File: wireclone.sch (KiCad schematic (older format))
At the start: 2 parts, among them P2 CONN_01X03, P3 CONN_01X03

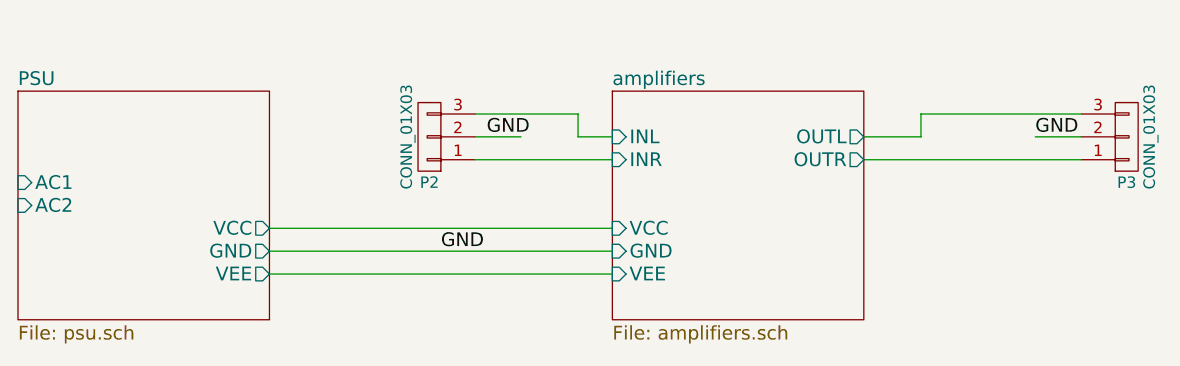
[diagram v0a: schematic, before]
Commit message: complete layout drafted
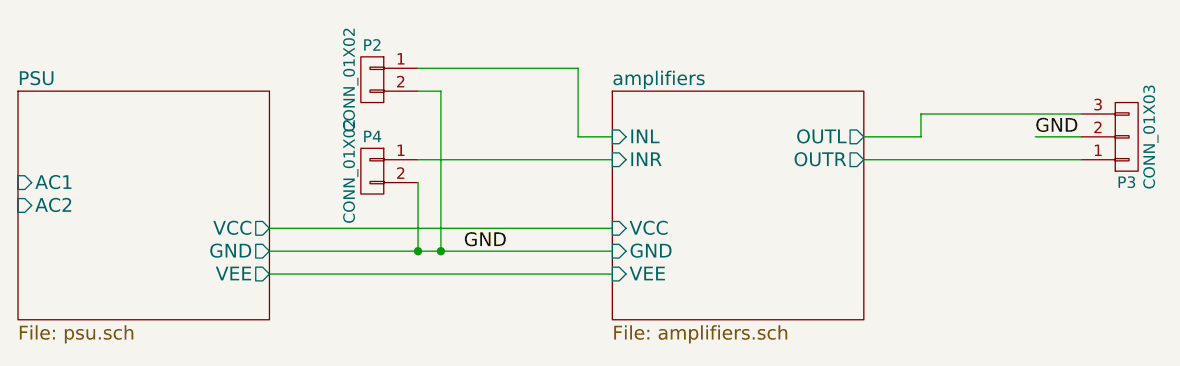
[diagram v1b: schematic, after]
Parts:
- removed P2: CONN_01X03, Pin_Headers:Pin_Header_Straight_1x03_Pitch2.54mm, symbol CONN_01X03
- added P2, P4: CONN_01X02, Pin_Headers:Pin_Header_Straight_1x02_Pitch2.54mm, symbol CONN_01X02
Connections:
- wire segments 13 -> 15
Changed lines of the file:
@@
 F6 "AC2" I L 4400 2400 60
 $EndSheet
-$Comp
-L CONN_01X03 P2
-U 1 1 584AA0FA
-P 6200 2100
-F 0 "P2" H 6200 2300 50  0000 C CNN
-F 1 "CONN_01X03" V 6300 2100 50  0000 C CNN
-F 2 "Pin_Headers:Pin_Header_Straight_1x03_Pitch2.54mm" H 6200 2100 50  0001 C CNN
-F 3 "" H 6200 2100 50  0000 C CNN
-	1    6200 2100
-	-1   0    0    1
-$EndComp
 Wire Wire Line
-	6400 2100 6600 2100
-Wire Wire Line
-	6400 2000 6850 2000
-Wire Wire Line
-	6850 2000 6850 2100
+	6850 1800 6850 2100
 $Comp
 L CONN_01X03 P3
@@
 GND
 Wire Wire Line
-	6400 2200 7000 2200
+	6150 2200 7000 2200
 Wire Wire Line
 	6850 2100 7000 2100
@@
 Wire Wire Line
 	5500 2700 7000 2700
-Text Label 6250 2600 0    60   ~ 0
+Text Label 6350 2600 0    60   ~ 0
 GND
-Text Label 6450 2100 0    60   ~ 0
-GND
+$Comp
+L CONN_01X02 P2
+U 1 1 59F1B351
+P 5950 1850
+F 0 "P2" H 5950 2000 50  0000 C CNN
+F 1 "CONN_01X02" V 6050 1850 50  0000 C CNN
+F 2 "Pin_Headers:Pin_Header_Straight_1x02_Pitch2.54mm" H 5950 1850 50  0001 C CNN
+F 3 "" H 5950 1850 50  0000 C CNN
+	1    5950 1850
+	-1   0    0    -1
+$EndComp
+$Comp
+L CONN_01X02 P4
+U 1 1 59F1B7BD
+P 5950 2250
+F 0 "P4" H 5950 2400 50  0000 C CNN
+F 1 "CONN_01X02" V 6050 2250 50  0000 C CNN
+F 2 "Pin_Headers:Pin_Header_Straight_1x02_Pitch2.54mm" H 5950 2250 50  0001 C CNN
+F 3 "" H 5950 2250 50  0000 C CNN
+	1    5950 2250
+	-1   0    0    -1
+$EndComp
+Wire Wire Line
+	6850 1800 6150 1800
+Wire Wire Line
+	6150 2600 6150 2300
+Connection ~ 6150 2600
+Wire Wire Line
+	6150 1900 6250 1900
+Wire Wire Line
+	6250 1900 6250 2600
+Connection ~ 6250 2600
 $EndSCHEMATC
